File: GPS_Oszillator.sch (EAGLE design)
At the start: 33 parts, among them IC1 74ACT04D, IC2 7805TV, X1 ST-SMB-V, X2 ST-SMB-V

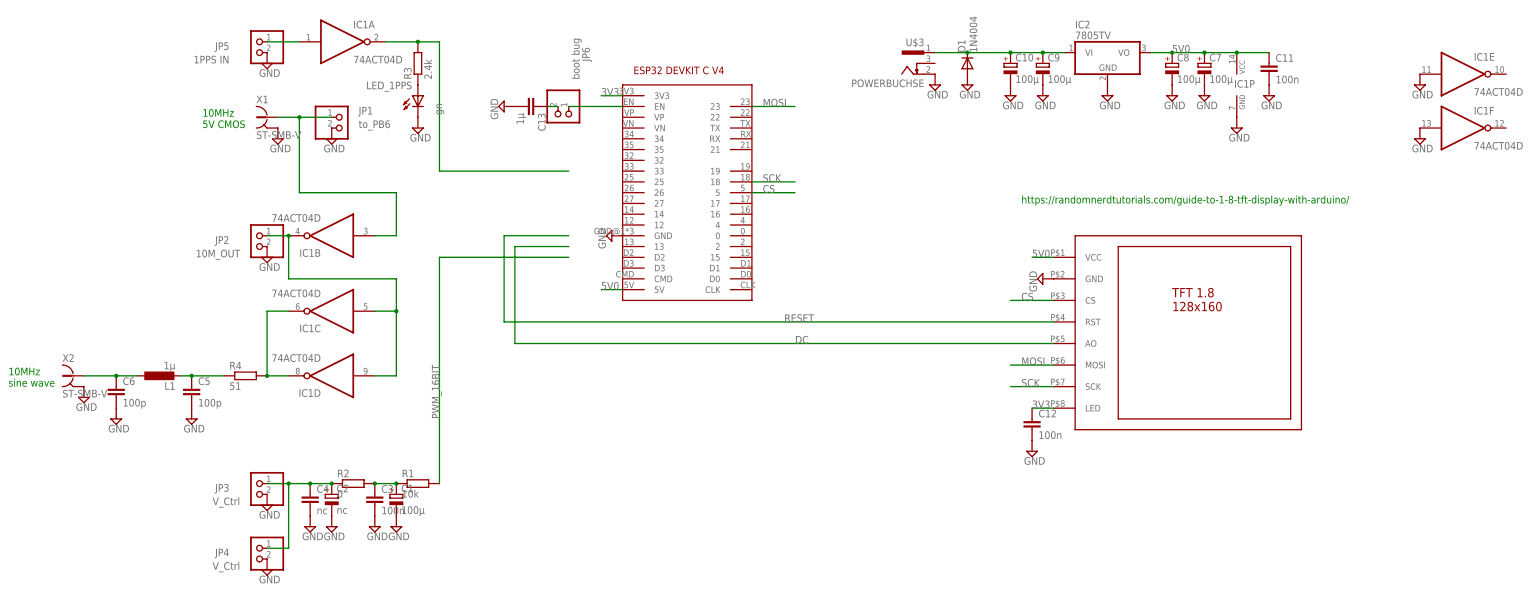
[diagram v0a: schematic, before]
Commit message: Add files via upload
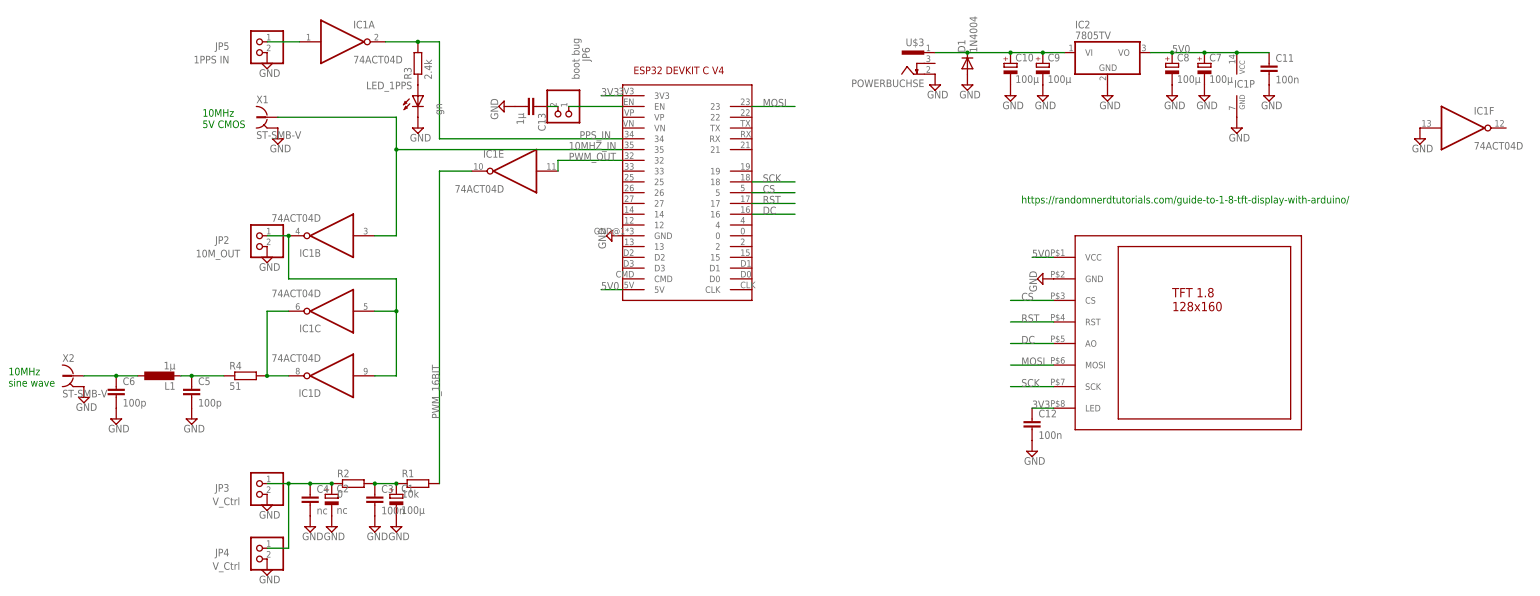
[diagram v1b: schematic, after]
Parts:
- removed JP1: to_PB6, pinhead:PINHD-1X2
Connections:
- removed net N$1: IC1A.O, R3.2
- removed net RESET: U$2.RST
- new net PPS_IN: IC1A.O, R3.2, U$4.34
- new net PWM_OUT: IC1E.I, U$4.32
- new net RST: U$2.RST, U$4.17
- net 10MHZ_IN: now also U$4.35; no longer JP1.1
- net DC: now also U$4.16
- net GND: no longer IC1E.I, JP1.2
- net PWM_16BIT: now also IC1E.O
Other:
- moved on the sheet: IC1E
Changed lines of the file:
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@@
 <part name="SUPPLY1" library="supply2" deviceset="GND" device=""/>
 <part name="IC2" library="linear" deviceset="78*" device="TV" technology="05"/>
-<part name="JP1" library="pinhead" deviceset="PINHD-1X2" device="" value="to_PB6"/>
-<part name="SUPPLY3" library="supply2" deviceset="GND" device=""/>
 <part name="JP2" library="pinhead" deviceset="PINHD-1X2" device="" value="10M_OUT"/>
 <part name="SUPPLY4" library="supply2" deviceset="GND" device=""/>
@@
 <part name="SUPPLY26" library="supply2" deviceset="GND" device=""/>
 <part name="SUPPLY25" library="supply2" deviceset="GND" device=""/>
-<part name="SUPPLY27" library="supply2" deviceset="GND" device=""/>
 <part name="D1" library="diode" deviceset="1N4004" device=""/>
 <part name="SUPPLY28" library="supply2" deviceset="GND" device=""/>
@@
 <instance part="IC1" gate="C" x="-68.58" y="33.02" rot="R180"/>
 <instance part="IC1" gate="D" x="-68.58" y="17.78" rot="R180"/>
-<instance part="IC1" gate="E" x="198.12" y="88.9"/>
+<instance part="IC1" gate="E" x="-25.4" y="66.04" rot="MR0"/>
 <instance part="IC1" gate="F" x="198.12" y="76.2"/>
 <instance part="IC1" gate="P" x="144.78" y="86.36"/>
@@
 <instance part="SUPPLY1" gate="GND" x="-81.28" y="73.66"/>
 <instance part="IC2" gate="A1" x="114.3" y="93.98"/>
-<instance part="JP1" gate="G$1" x="-66.04" y="76.2" smashed="yes">
-<attribute name="NAME" x="-62.23" y="79.375" size="1.778" layer="95"/>
-<attribute name="VALUE" x="-62.23" y="76.2" size="1.778" layer="96"/>
-</instance>
-<instance part="SUPPLY3" gate="GND" x="-68.58" y="73.66"/>
 <instance part="JP2" gate="G$1" x="-86.36" y="48.26" smashed="yes" rot="MR0">
 <attribute name="NAME" x="-92.71" y="48.895" size="1.778" layer="95" rot="MR0"/>
@@
 <instance part="SUPPLY26" gate="GND" x="73.66" y="86.36"/>
 <instance part="SUPPLY25" gate="GND" x="187.96" y="73.66"/>
-<instance part="SUPPLY27" gate="GND" x="187.96" y="86.36"/>
 <instance part="D1" gate="1" x="81.28" y="91.44" rot="R90"/>
 <instance part="SUPPLY28" gate="GND" x="81.28" y="86.36"/>
@@
 </segment>
 <segment>
-<pinref part="JP1" gate="G$1" pin="2"/>
-<pinref part="SUPPLY3" gate="GND" pin="GND"/>
-</segment>
-<segment>
 <pinref part="JP2" gate="G$1" pin="2"/>
 <pinref part="SUPPLY4" gate="GND" pin="GND"/>
@@
 </segment>
 <segment>
-<pinref part="IC1" gate="E" pin="I"/>
-<pinref part="SUPPLY27" gate="GND" pin="GND"/>
-</segment>
-<segment>
 <pinref part="D1" gate="1" pin="A"/>
 <pinref part="SUPPLY28" gate="GND" pin="GND"/>
@@
 </segment>
 </net>
-<net name="N$1" class="0">
+<net name="PPS_IN" class="0">
 <segment>
 <pinref part="IC1" gate="A" pin="O"/>
 <wire x1="-55.88" y1="96.52" x2="-48.26" y2="96.52" width="0.1524" layer="91"/>
 <wire x1="-48.26" y1="96.52" x2="-43.18" y2="96.52" width="0.1524" layer="91"/>
-<wire x1="-43.18" y1="96.52" x2="-43.18" y2="66.04" width="0.1524" layer="91"/>
-<wire x1="-43.18" y1="66.04" x2="-12.7" y2="66.04" width="0.1524" layer="91"/>
+<wire x1="-43.18" y1="96.52" x2="-43.18" y2="73.66" width="0.1524" layer="91"/>
 <pinref part="R3" gate="G$1" pin="2"/>
 <junction x="-48.26" y="96.52"/>
+<pinref part="U$4" gate="G$1" pin="34"/>
+<wire x1="0" y1="73.66" x2="-43.18" y2="73.66" width="0.1524" layer="91"/>
+<label x="-10.16" y="73.66" size="1.778" layer="95"/>
 </segment>
 </net>
@@
 <segment>
 <pinref part="X1" gate="G1" pin="1"/>
-<pinref part="JP1" gate="G$1" pin="1"/>
-<wire x1="-81.28" y1="78.74" x2="-76.2" y2="78.74" width="0.1524" layer="91"/>
-<wire x1="-76.2" y1="78.74" x2="-68.58" y2="78.74" width="0.1524" layer="91"/>
-<wire x1="-76.2" y1="78.74" x2="-76.2" y2="60.96" width="0.1524" layer="91"/>
-<wire x1="-76.2" y1="60.96" x2="-53.34" y2="60.96" width="0.1524" layer="91"/>
-<wire x1="-53.34" y1="60.96" x2="-53.34" y2="50.8" width="0.1524" layer="91"/>
+<wire x1="-81.28" y1="78.74" x2="-53.34" y2="78.74" width="0.1524" layer="91"/>
+<wire x1="-53.34" y1="78.74" x2="-53.34" y2="71.12" width="0.1524" layer="91"/>
 <pinref part="IC1" gate="B" pin="I"/>
+<wire x1="-53.34" y1="71.12" x2="-53.34" y2="50.8" width="0.1524" layer="91"/>
 <wire x1="-53.34" y1="50.8" x2="-58.42" y2="50.8" width="0.1524" layer="91"/>
-<junction x="-76.2" y="78.74"/>
+<pinref part="U$4" gate="G$1" pin="35"/>
+<wire x1="0" y1="71.12" x2="-53.34" y2="71.12" width="0.1524" layer="91"/>
+<junction x="-53.34" y="71.12"/>
+<label x="-12.7" y="71.12" size="1.778" layer="95"/>
 </segment>
 </net>
@@
 <segment>
 <pinref part="R1" gate="G$1" pin="2"/>
-<wire x1="-43.18" y1="-7.62" x2="-43.18" y2="45.72" width="0.1524" layer="91"/>
-<wire x1="-12.7" y1="45.72" x2="-43.18" y2="45.72" width="0.1524" layer="91"/>
+<wire x1="-43.18" y1="-7.62" x2="-43.18" y2="66.04" width="0.1524" layer="91"/>
+<wire x1="-35.56" y1="66.04" x2="-43.18" y2="66.04" width="0.1524" layer="91"/>
 <label x="-43.18" y="7.62" size="1.778" layer="95" rot="R90"/>
+<pinref part="IC1" gate="E" pin="O"/>
 </segment>
 </net>
@@
 </segment>
 </net>
-<net name="RESET" class="0">
-<segment>
-<wire x1="-12.7" y1="50.8" x2="-27.94" y2="50.8" width="0.1524" layer="91"/>
-<wire x1="-27.94" y1="50.8" x2="-27.94" y2="30.48" width="0.1524" layer="91"/>
-<wire x1="-27.94" y1="30.48" x2="101.6" y2="30.48" width="0.1524" layer="91"/>
-<label x="38.1" y="30.48" size="1.778" layer="95"/>
+<net name="RST" class="0">
+<segment>
+<wire x1="91.44" y1="30.48" x2="101.6" y2="30.48" width="0.1524" layer="91"/>
 <pinref part="U$2" gate="G$1" pin="RST"/>
+<label x="93.98" y="30.48" size="1.778" layer="95"/>
+</segment>
+<segment>
+<wire x1="30.48" y1="58.42" x2="40.64" y2="58.42" width="0.1524" layer="91"/>
+<label x="33.02" y="58.42" size="1.778" layer="95"/>
+<pinref part="U$4" gate="G$1" pin="17"/>
 </segment>
 </net>
 <net name="DC" class="0">
 <segment>
-<wire x1="-12.7" y1="48.26" x2="-25.4" y2="48.26" width="0.1524" layer="91"/>
-<wire x1="-25.4" y1="48.26" x2="-25.4" y2="25.4" width="0.1524" layer="91"/>
-<wire x1="-25.4" y1="25.4" x2="101.6" y2="25.4" width="0.1524" layer="91"/>
-<label x="40.64" y="25.4" size="1.778" layer="95"/>
+<wire x1="91.44" y1="25.4" x2="101.6" y2="25.4" width="0.1524" layer="91"/>
 <pinref part="U$2" gate="G$1" pin="AO"/>
+<label x="93.98" y="25.4" size="1.778" layer="95"/>
+</segment>
+<segment>
+<wire x1="30.48" y1="55.88" x2="40.64" y2="55.88" width="0.1524" layer="91"/>
+<label x="33.02" y="55.88" size="1.778" layer="95"/>
+<pinref part="U$4" gate="G$1" pin="16"/>
 </segment>
 </net>
@@
 </segment>
 </net>
+<net name="PWM_OUT" class="0">
+<segment>
+<pinref part="IC1" gate="E" pin="I"/>
+<wire x1="-15.24" y1="66.04" x2="-15.24" y2="68.58" width="0.1524" layer="91"/>
+<pinref part="U$4" gate="G$1" pin="32"/>
+<wire x1="-15.24" y1="68.58" x2="0" y2="68.58" width="0.1524" layer="91"/>
+<label x="-12.7" y="68.58" size="1.778" layer="95"/>
+</segment>
+</net>
